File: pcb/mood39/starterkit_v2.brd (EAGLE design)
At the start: 32 x 32 mm, 17 parts, among them IC1 TINY85, IC2 LM2940, X1 PWRUSB, X3 PWRUNREG

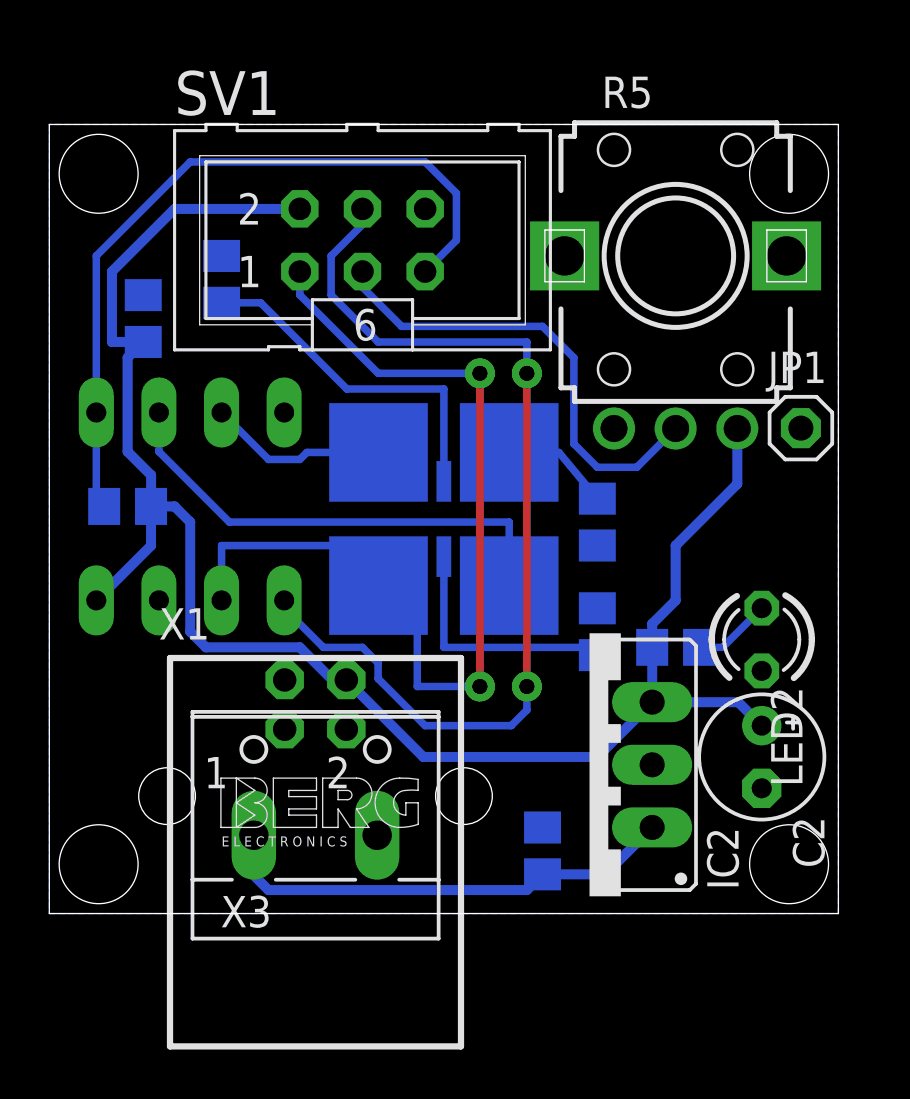
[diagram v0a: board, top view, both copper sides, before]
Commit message: commit before battery low
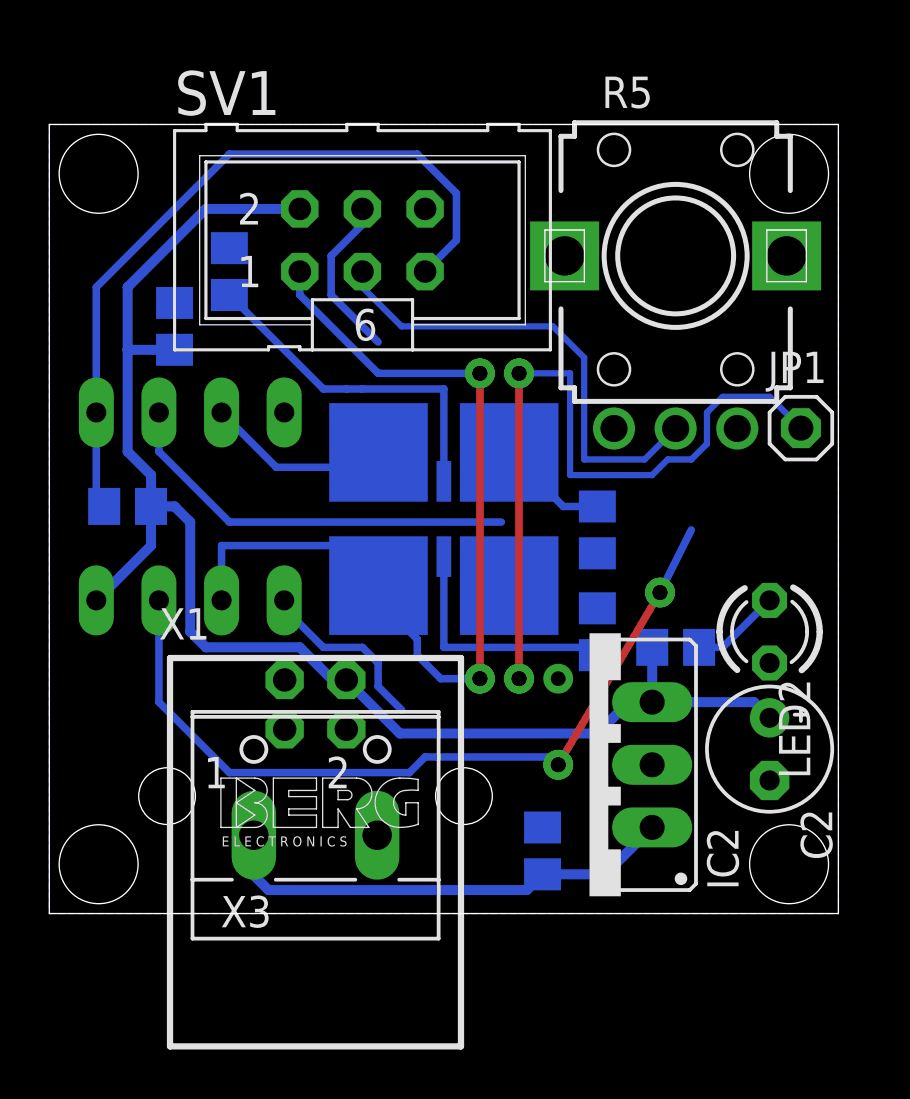
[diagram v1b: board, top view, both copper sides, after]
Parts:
- moved C1 1.31 mm to (5.08, 23.8)
- moved C2 0.45 mm to (29.2, 6.67)
- moved LED2 0.45 mm to (29.2, 11.4)
- moved R2 0.45 mm to (7.30, 26.0)
- moved R4 0.32 mm to (22.2, 15.6)
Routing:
- net SCK: track 19.1 -> 52.0 mm, vias 0 -> 2
- net VCC: track 70.3 -> 58.7 mm
- net MOSI: track 40.4 -> 44.6 mm
- net PB3: track 19.6 -> 16.7 mm
- net MISO: track 40.7 -> 42.1 mm
